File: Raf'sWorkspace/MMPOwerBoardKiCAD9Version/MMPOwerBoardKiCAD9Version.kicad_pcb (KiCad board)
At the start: 2 copper layers, 77.5 x 59 mm, 102 parts, among them J1 TYPE-C-31-M-04, J2 Conn_02x16_Odd_Even, J3 Conn_01x02, Q1 SS8050, SW1 SS-12D11-G050, U1 HUSB237, U10 TPS22917DBVR, U11 AMS1117-5.0, U2 TP4056-42-ESOP8, U3 DRV8833PWPR, U4 TPS63802DLAR, U5 TPS22917DBVR, U6 TPS61236PRWLR, U7 INA219AIDR, U9 DRV8833PWPR

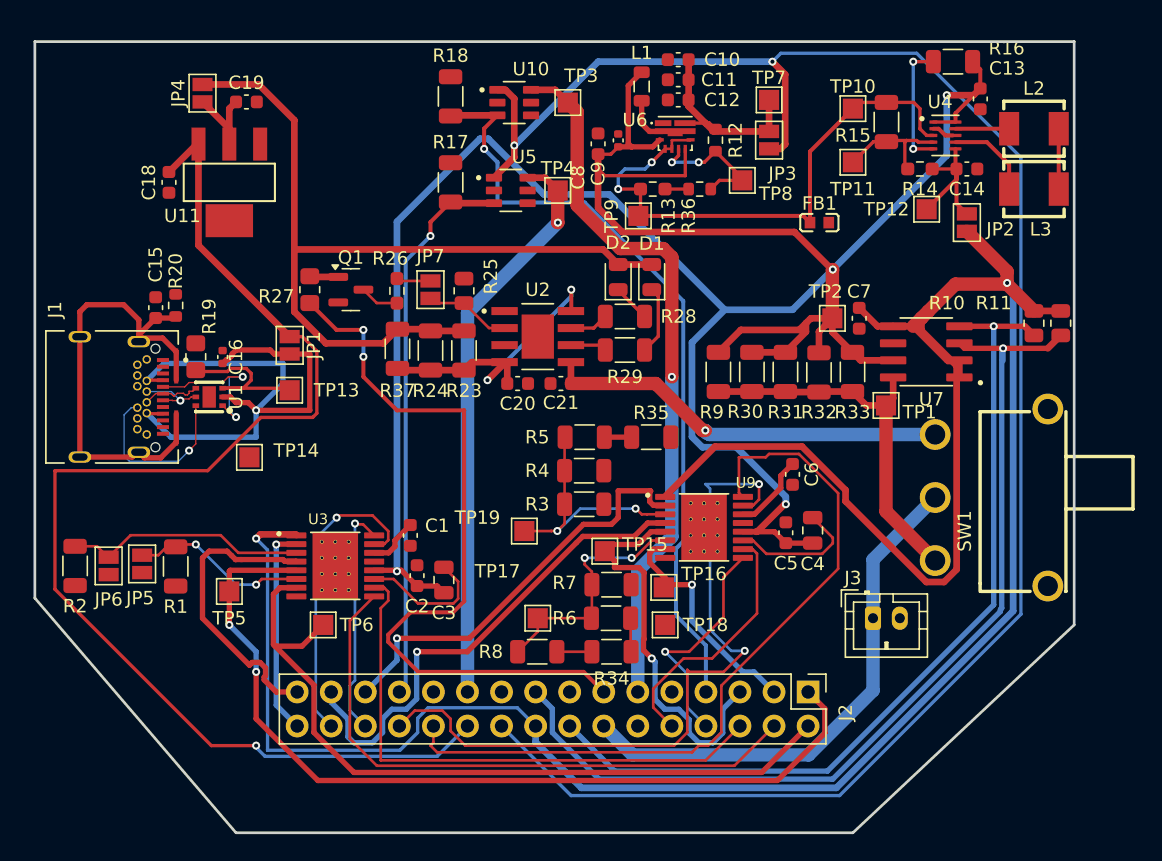
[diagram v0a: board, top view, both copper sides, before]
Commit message: PCB seems to be done - BOM also generated
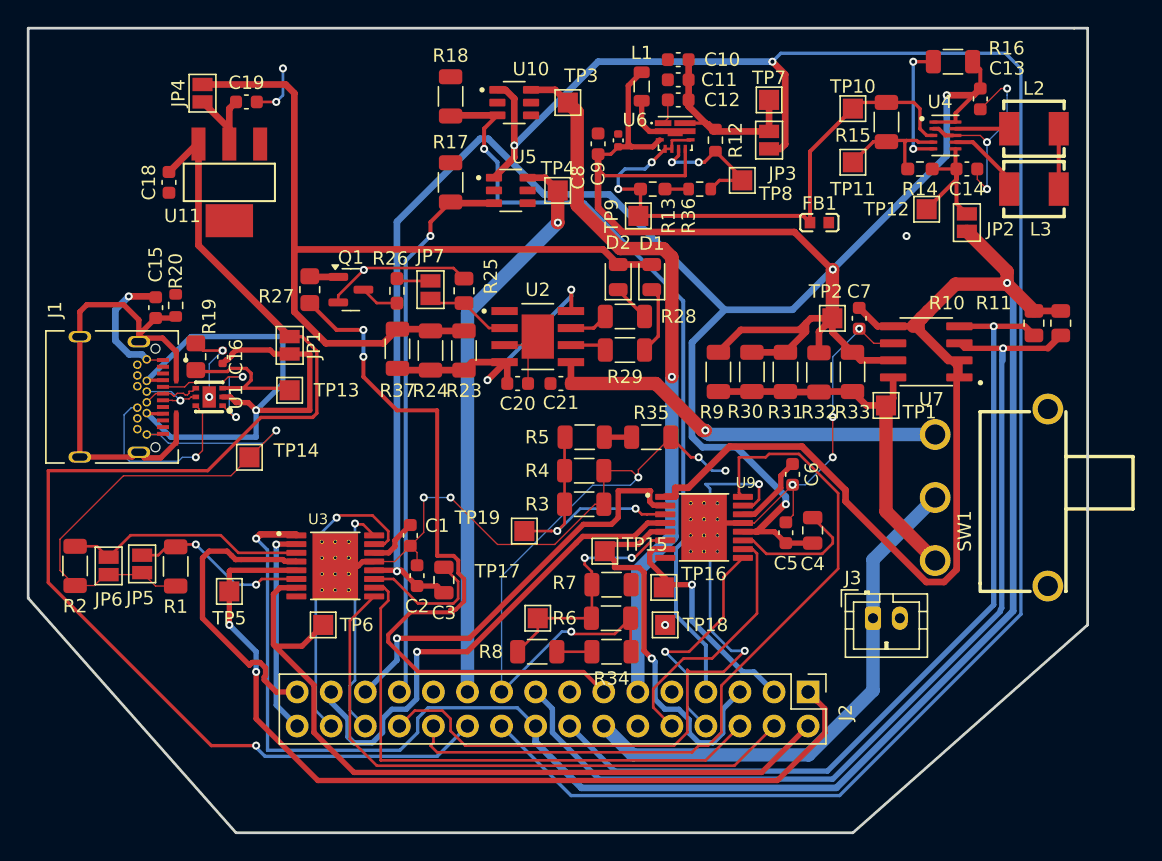
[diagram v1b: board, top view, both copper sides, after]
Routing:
- net GND: track 4.17 -> 206.9 mm, vias 0 -> 22
- net /5V: track 140.3 -> 144.2 mm
- net Net-(JP1-B): track 46.5 -> 49.4 mm
- net /5V_charge: track 63.5 -> 64.6 mm
- net Net-(J1-CC2): track 13.2 -> 14.3 mm
- net /9V: track 94.4 -> 95.1 mm
- net Net-(U4-L2): track 6.53 -> 5.92 mm
- added copper zone on B.Cu, net GND
- added copper zone on F.Cu, net GND
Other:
- board size 77.5 x 59 mm -> 79 x 60 mm
